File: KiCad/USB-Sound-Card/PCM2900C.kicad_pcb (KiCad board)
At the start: 2 copper layers, 21 parts, among them J101 USB_C_Receptacle_USB2.0, J2 Conn_01x03_Male, U101 PCM2900C, Y1 12MHz 18pF

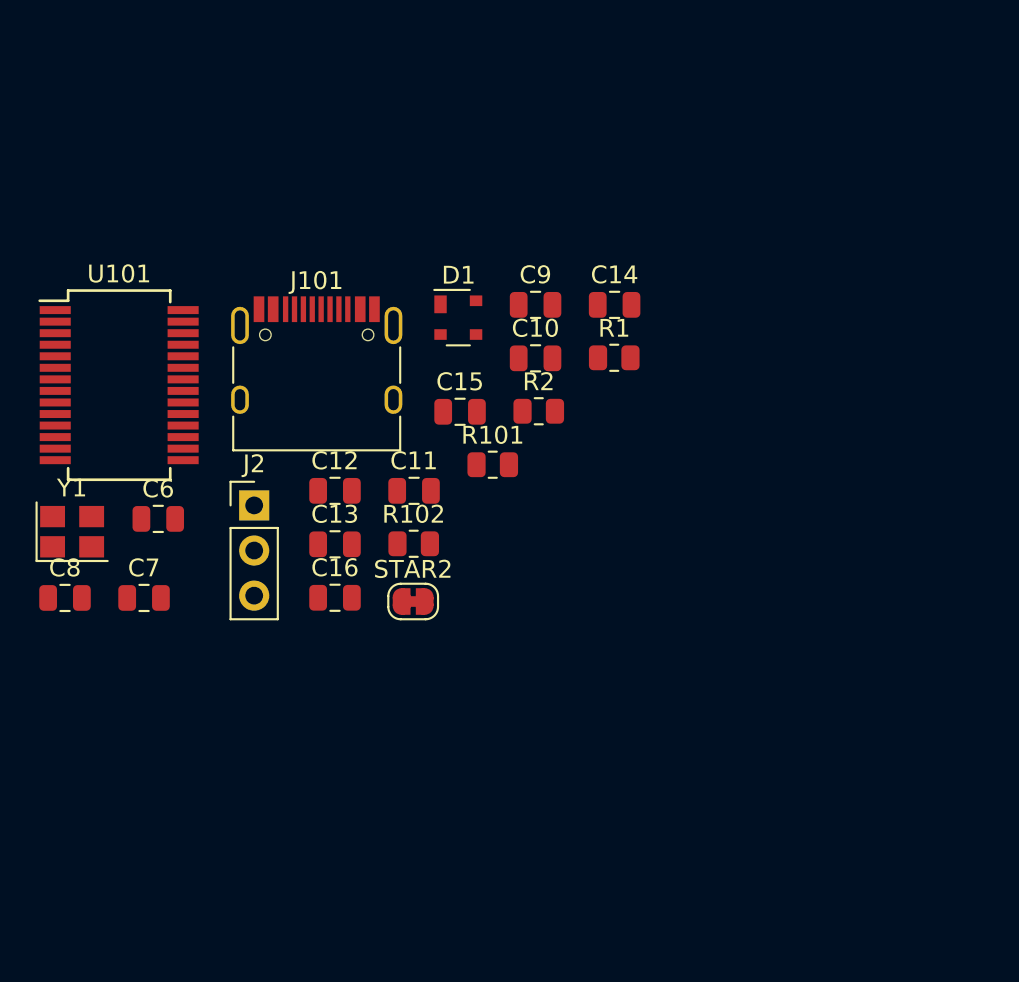
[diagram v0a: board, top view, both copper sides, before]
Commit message: hastily slapped together pcb
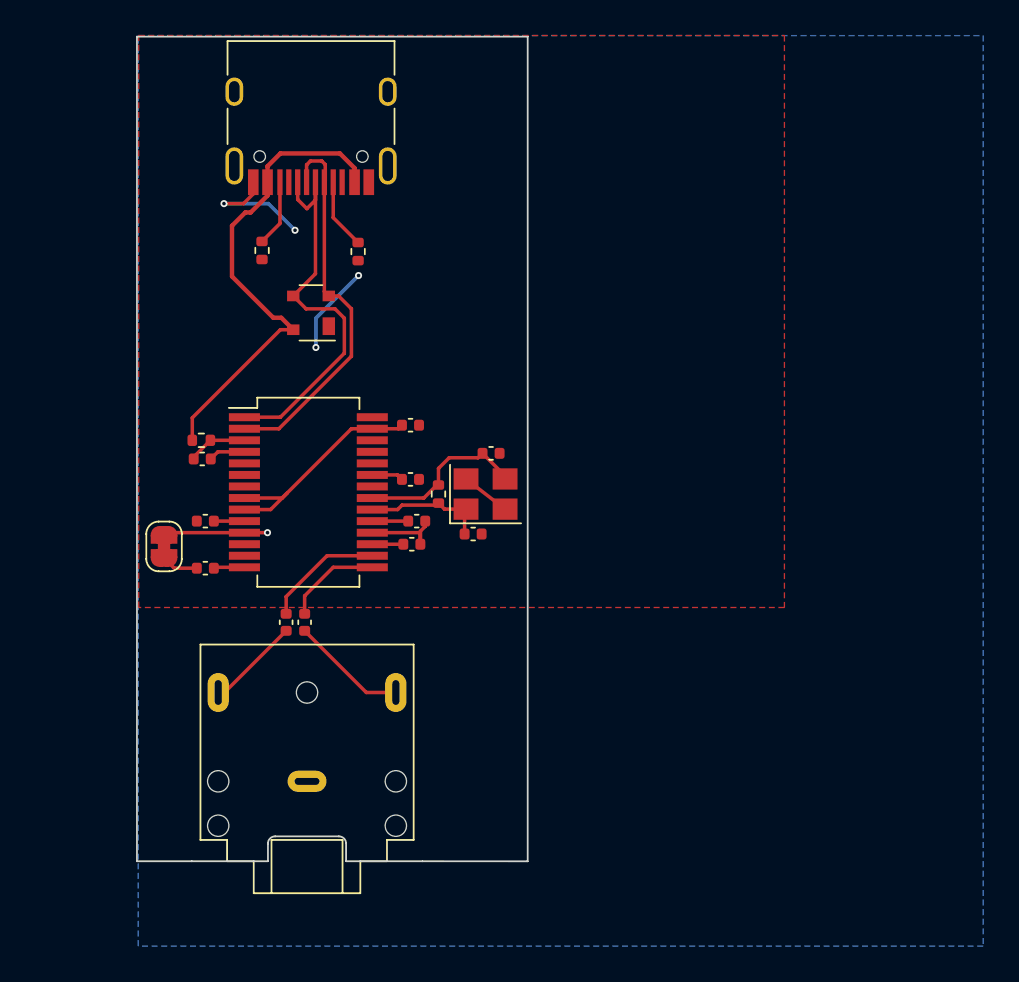
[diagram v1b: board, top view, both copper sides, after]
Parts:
- removed J2: Conn_01x03_Male, Connector_PinHeader_2.54mm:PinHeader_1x03_P2.54mm_Vertical
- added J102: AudioJack3, Connector_Audio:Jack_3.5mm_CUI_SJ1-3523N_Horizontal, F.Cu at (43.2, 57.2)
- C10, C11, C12, C13, C14, C15, C16, C6, C7, C8, C9: footprint Capacitor_SMD:C_0805_2012Metric -> Capacitor_SMD:C_0402_1005Metric
- R1, R101, R102, R2: footprint Resistor_SMD:R_0805_2012Metric -> Resistor_SMD:R_0402_1005Metric
- moved C14 25.0 mm to (43.0, 48.2), turned to -90 degrees
- moved Y1 23.4 mm to (53.2, 41.0)
- moved R2 19.1 mm to (37.2, 38.0)
- moved R102 18.6 mm to (40.6, 27.3), turned to -90 degrees
- moved J101 15.2 mm to (43.4, 19.4), turned to 180 degrees
- moved STAR2 14.4 mm to (35.1, 44.0), turned to 90 degrees
- moved R101 14.2 mm to (46.0, 27.4), turned to -90 degrees
- moved R1 12.5 mm to (50.6, 41.0), turned to -90 degrees
- moved U101 12.2 mm to (43.2, 40.9)
- moved C16 12.0 mm to (53.5, 38.7)
- moved C10 9.80 mm to (49.0, 40.2)
- moved C9 9.77 mm to (49.0, 37.1)
- moved D1 8.29 mm to (43.4, 30.8), turned to 180 degrees
- moved C8 8.08 mm to (37.5, 45.2), turned to 180 degrees
- moved C15 6.92 mm to (52.5, 43.2)
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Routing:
- net VBUS: track 0.00 -> 27.2 mm
- net AGNDP: track 0.00 -> 23.9 mm, vias 0 -> 4
- net USB D+: track 0.00 -> 22.8 mm
- net USB D-: track 0.00 -> 21.6 mm
- net Net-(C9-Pad1): track 0.00 -> 13.3 mm
- net Net-(C16-Pad1): track 0.00 -> 9.50 mm
- net VOUTL: track 0.00 -> 6.77 mm
- net Net-(C15-Pad1): track 0.00 -> 6.73 mm
- net /L-USB-In: track 0.00 -> 6.57 mm
- net AGNDC: track 0.00 -> 5.70 mm, vias 0 -> 1
- net VOUTR: track 0.00 -> 5.48 mm
- net /R-USB-In: track 0.00 -> 4.91 mm
- net Net-(J101-PadA5): track 0.00 -> 3.97 mm
- net Net-(J101-PadB5): track 0.00 -> 3.75 mm
- net Net-(C6-Pad1): track 0.00 -> 3.24 mm
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- added copper zone on B.Cu, net AGNDC
- added copper zone on F.Cu, net AGNDP
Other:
- board outline added: 22 x 46.4 mm
